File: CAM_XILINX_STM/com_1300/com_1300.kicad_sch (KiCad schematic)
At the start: 124 parts, among them J2 9-68RD-0.635SF, J3 MEC1-108-01-S-D-RA1-SL, J4 Conn_02x10_Top_Bottom, U1 LT1963AxST-3.3, U17 MT48LC16M16A2TG-7E, U2 STM32F415RGTx, U3 AM29LV320DT90EC, U4 TC74LCX373FT, U6 LP3982IMM-ADJ, U7 LTC3411EMS, Y1 16mHz, Y2 40mHZ

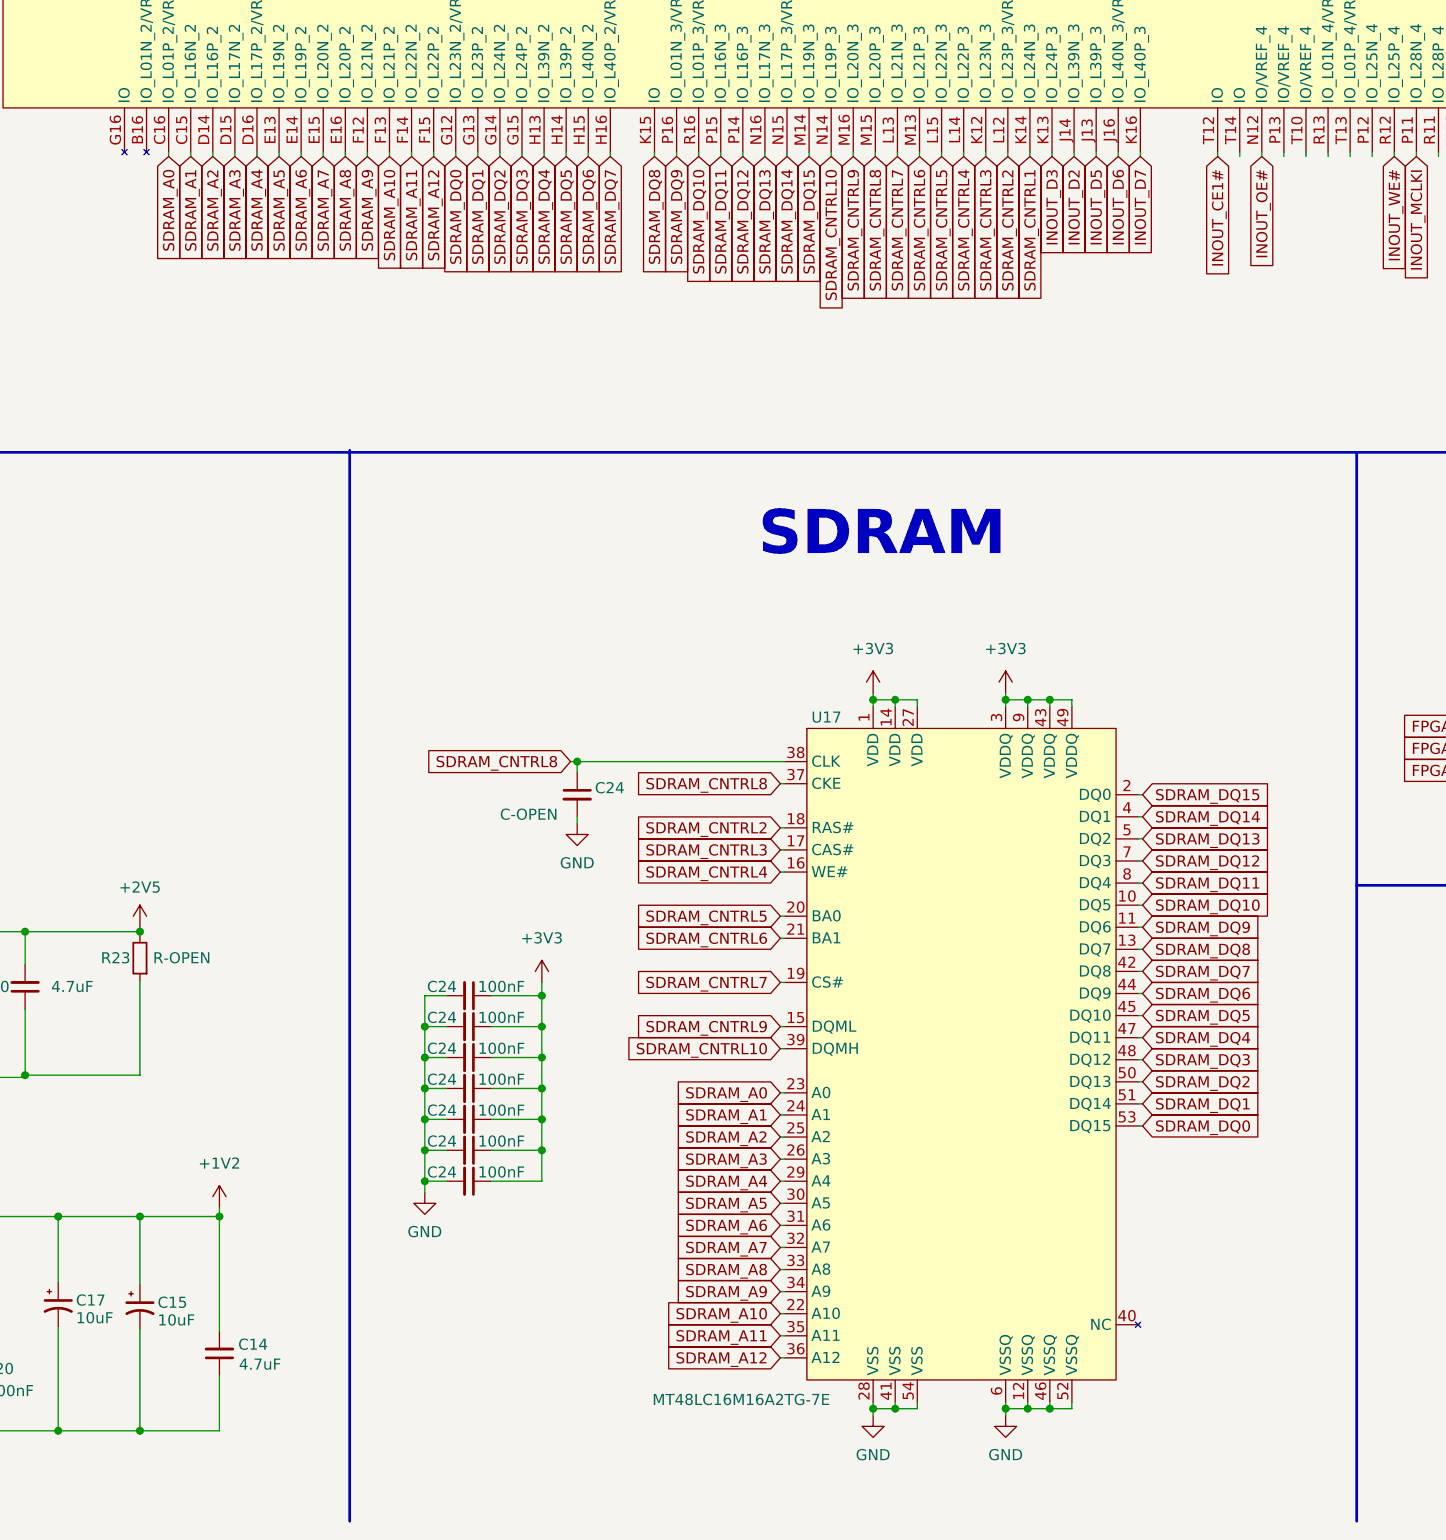
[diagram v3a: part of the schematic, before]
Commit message: 22323
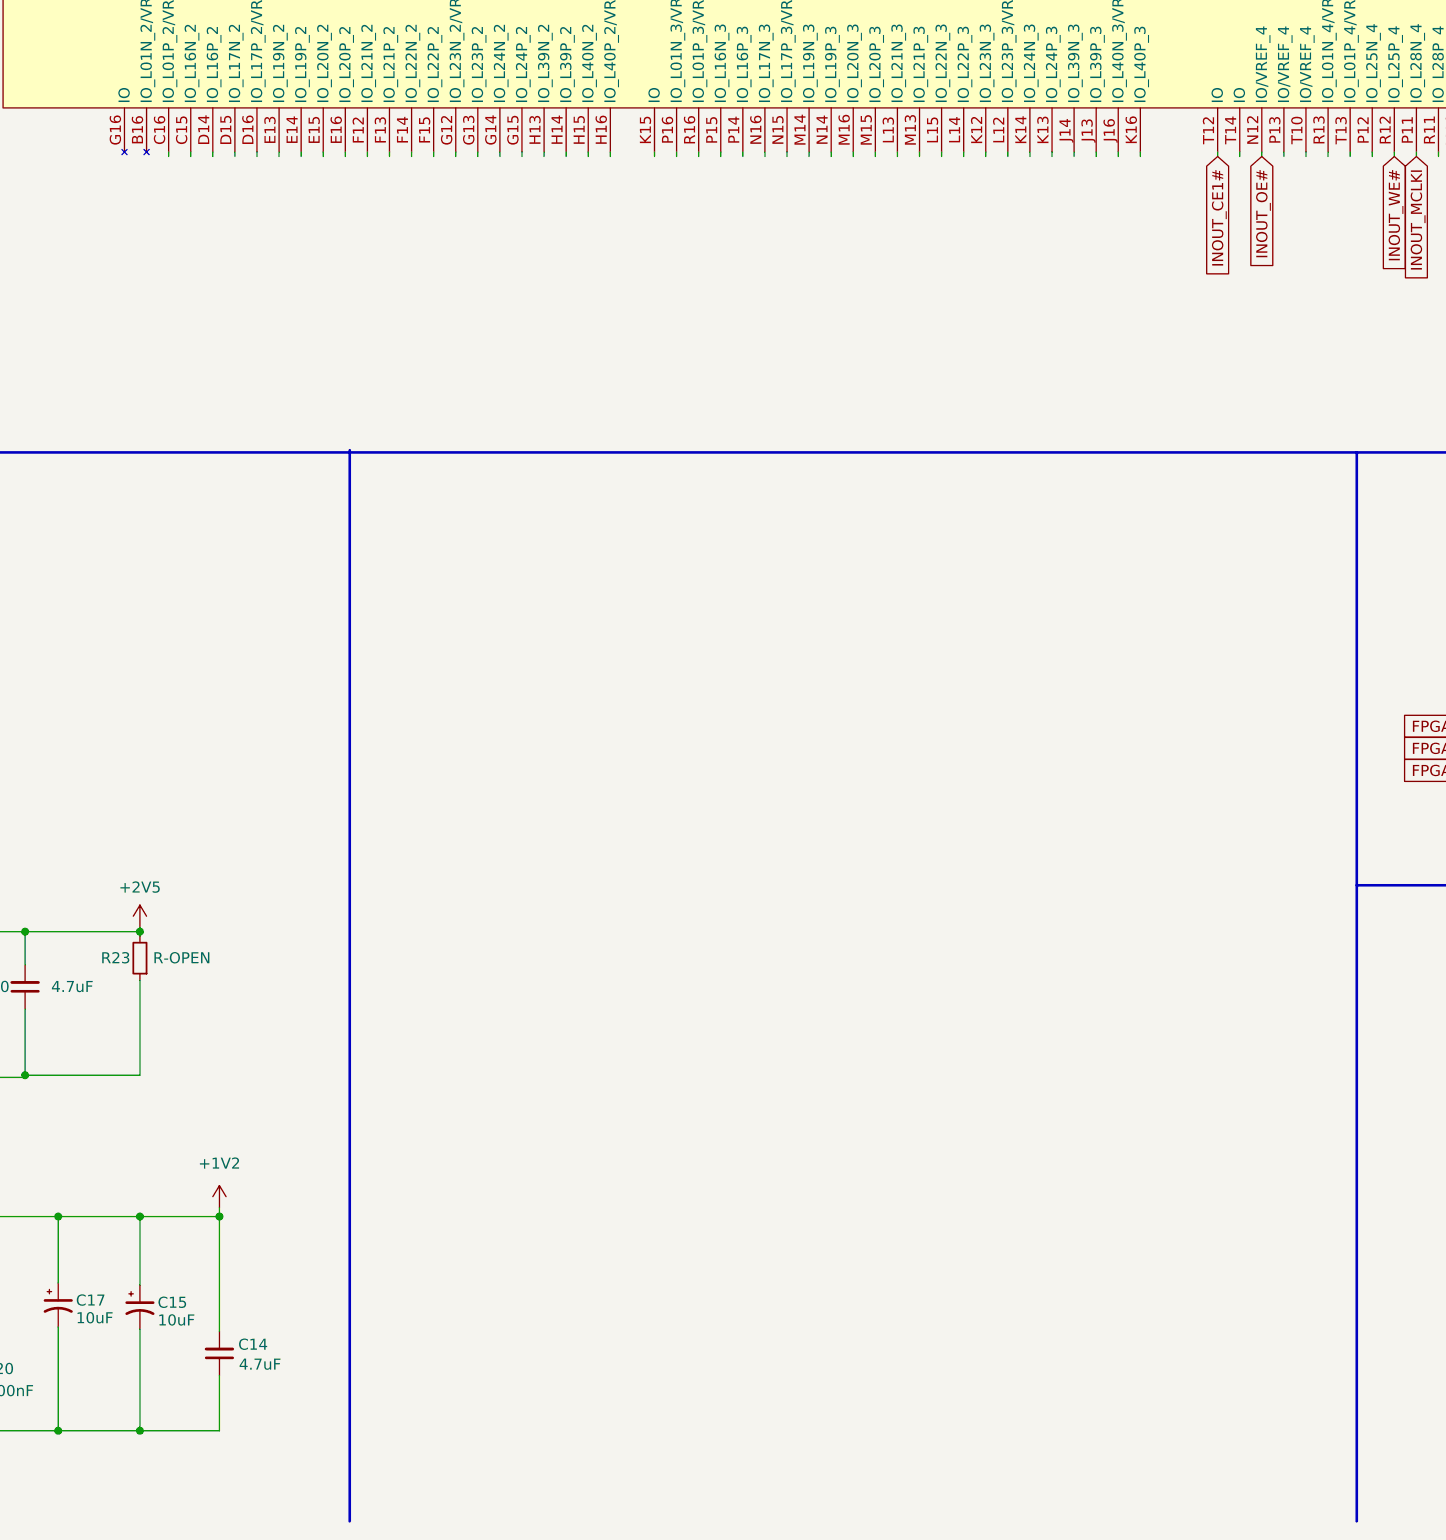
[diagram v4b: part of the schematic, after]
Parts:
- removed C24 (x8): C-OPEN, Capacitor_SMD:C_0603_1608Metric, symbol Device:C_Small
- removed U17: MT48LC16M16A2TG-7E, Package_SO:TSOP-II-54_22.2x10.16mm_P0.8mm, symbol Storage:MT48LC16M16A2TG-7E
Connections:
- net INOUT_D2: no longer U.J14 (IO_L39N_3)
- net INOUT_D3: no longer U.K13 (IO_L24P_3)
- net INOUT_D5: no longer U.J13 (IO_L39P_3)
- net INOUT_D6: no longer U.J16 (IO_L40N_3/VREF_3)
- net INOUT_D7: no longer U.K16 (IO_L40P_3)
- net SDRAM_A0: no longer names the net of U.C16 (IO_L01P_2/VRN_2)
- net SDRAM_A1: no longer names the net of U.C15 (IO_L16N_2)
- net SDRAM_A10: no longer names the net of U.F13 (IO_L21P_2)
- net SDRAM_A11: no longer names the net of U.F14 (IO_L22N_2)
- net SDRAM_A12: no longer names the net of U.F15 (IO_L22P_2)
- net SDRAM_A2: no longer names the net of U.D14 (IO_L16P_2)
- net SDRAM_A3: no longer names the net of U.D15 (IO_L17N_2)
- net SDRAM_A4: no longer names the net of U.D16 (IO_L17P_2/VREF_2)
- net SDRAM_A5: no longer names the net of U.E13 (IO_L19N_2)
- net SDRAM_A6: no longer names the net of U.E14 (IO_L19P_2)
- net SDRAM_A7: no longer names the net of U.E15 (IO_L20N_2)
- net SDRAM_A8: no longer names the net of U.E16 (IO_L20P_2)
- net SDRAM_A9: no longer names the net of U.F12 (IO_L21N_2)
- net SDRAM_CNTRL1: no longer names the net of U.K14 (IO_L24N_3)
- net SDRAM_CNTRL10: no longer names the net of U.N14 (IO_L19P_3)
- net SDRAM_CNTRL2: no longer names the net of U.L12 (IO_L23P_3/VREF_3)
- net SDRAM_CNTRL3: no longer names the net of U.K12 (IO_L23N_3)
- net SDRAM_CNTRL4: no longer names the net of U.L14 (IO_L22P_3)
- net SDRAM_CNTRL5: no longer names the net of U.L15 (IO_L22N_3)
- net SDRAM_CNTRL6: no longer names the net of U.M13 (IO_L21P_3)
- net SDRAM_CNTRL7: no longer names the net of U.L13 (IO_L21N_3)
- net SDRAM_CNTRL8: no longer names the net of U.M15 (IO_L20P_3)
- net SDRAM_CNTRL9: no longer names the net of U.M16 (IO_L20N_3)
- net SDRAM_DQ0: no longer names the net of U.G12 (IO_L23N_2/VREF_2)
- net SDRAM_DQ1: no longer names the net of U.G13 (IO_L23P_2)
- net SDRAM_DQ10: no longer names the net of U.R16 (IO_L01P_3/VRN_3)
- net SDRAM_DQ11: no longer names the net of U.P15 (IO_L16N_3)
- net SDRAM_DQ12: no longer names the net of U.P14 (IO_L16P_3)
- net SDRAM_DQ13: no longer names the net of U.N16 (IO_L17N_3)
- net SDRAM_DQ14: no longer names the net of U.N15 (IO_L17P_3/VREF_3)
- net SDRAM_DQ15: no longer names the net of U.M14 (IO_L19N_3)
- net SDRAM_DQ2: no longer names the net of U.G14 (IO_L24N_2)
- net SDRAM_DQ3: no longer names the net of U.G15 (IO_L24P_2)
- net SDRAM_DQ4: no longer names the net of U.H13 (IO_L39N_2)
- net SDRAM_DQ5: no longer names the net of U.H14 (IO_L39P_2)
- net SDRAM_DQ6: no longer names the net of U.H15 (IO_L40N_2)
- net SDRAM_DQ7: no longer names the net of U.H16 (IO_L40P_2/VREF_2)
- net SDRAM_DQ8: no longer names the net of U.K15 (IO)
- net SDRAM_DQ9: no longer names the net of U.P16 (IO_L01N_3/VRP_3)
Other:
- note removed: "SDRAM"
